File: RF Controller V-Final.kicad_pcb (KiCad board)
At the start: 2 copper layers, 132 x 67.5 mm, 38 parts, among them J2 J_OLED, J3 BAT+, J4 BAT-, SW1 EG1218, U1 Teensy4.0, U3 NRF24L01, U5 AP2112K-3.3, U7 Pitch/Roll, U8 TPS542025DDCR, U9 Throttle/Yaw

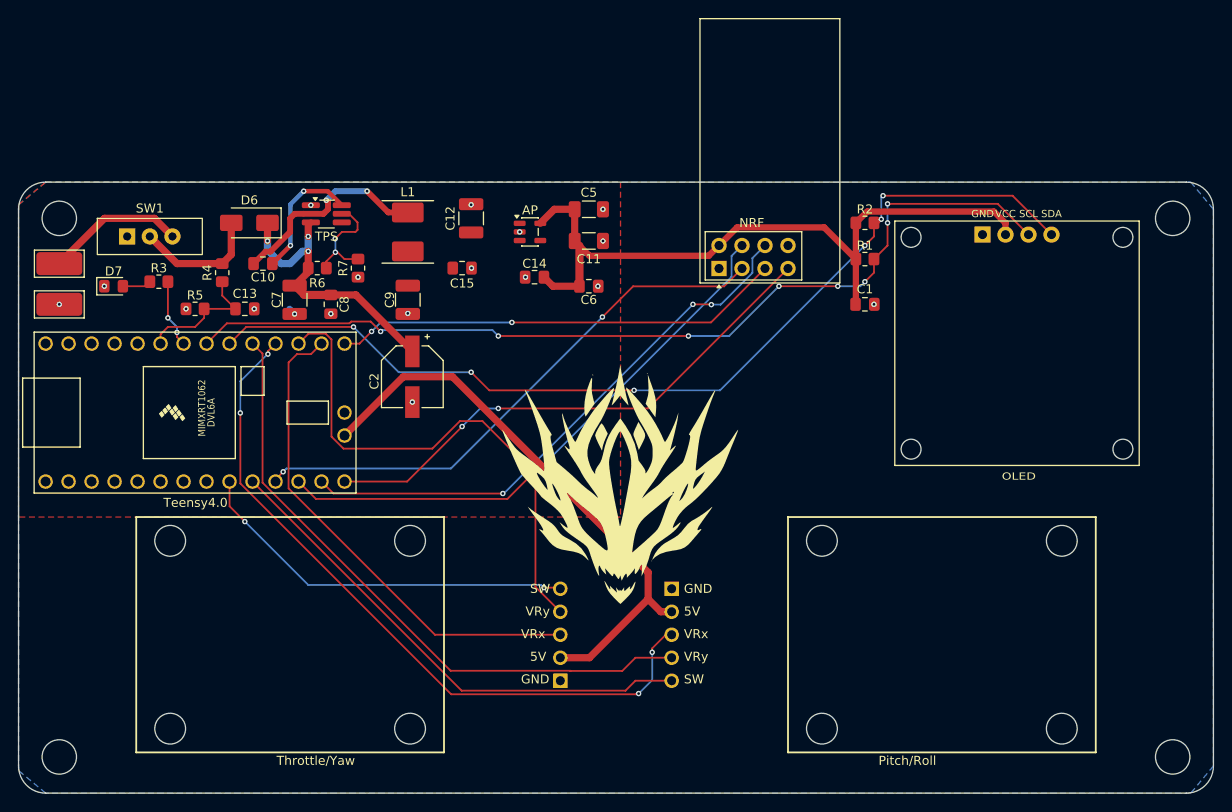
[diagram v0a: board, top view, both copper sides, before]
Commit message: Edited positions
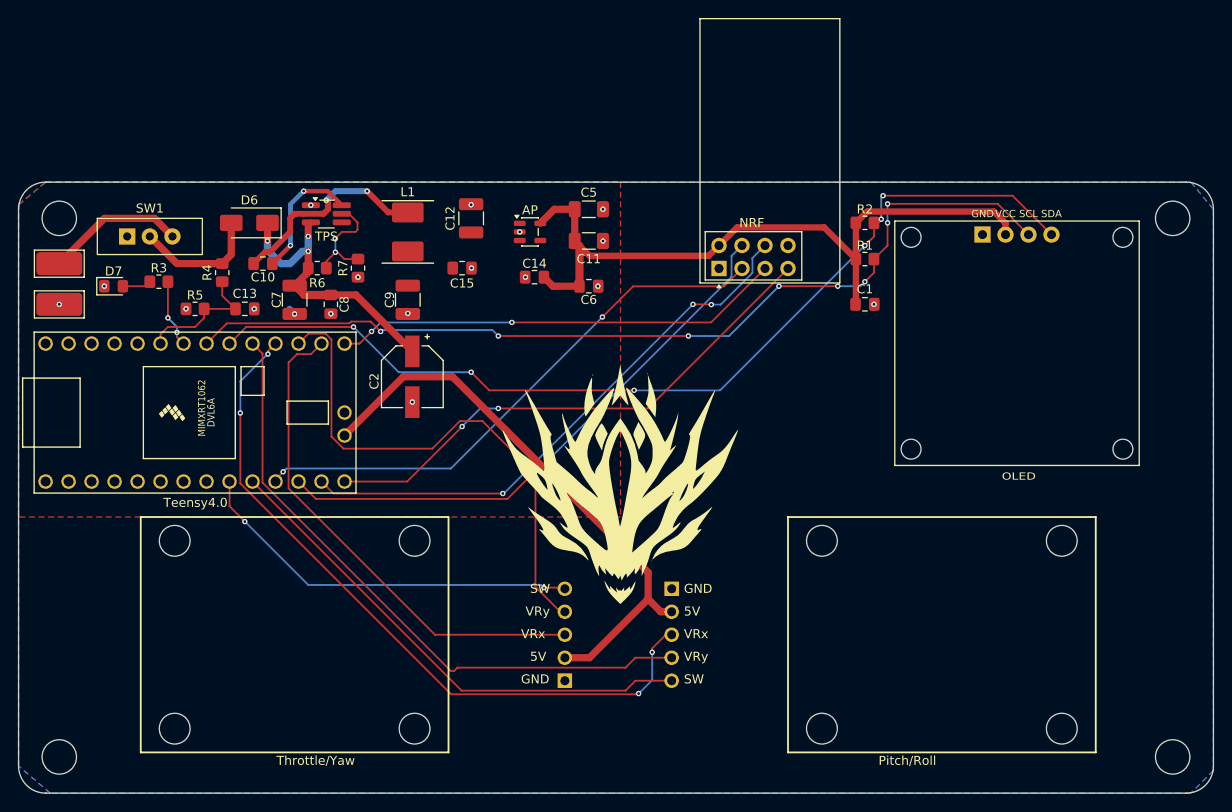
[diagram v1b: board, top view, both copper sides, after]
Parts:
- moved U9 0.50 mm to (129.5, 105.0)
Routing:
- net /D9: track 43.0 -> 44.0 mm
- net /3v3: track 63.7 -> 63.2 mm
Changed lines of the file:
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@@
 	(footprint "JOYYFOOT:JOY1"
 		(layer "F.Cu")
-		(at 129 105 180)
+		(at 129.5 105 180)
 		(property "Reference" "U9"
 			(at 10.73 -10.66 180)
@@
 	)
 	(segment
-		(start 140.039265 112.800735)
-		(end 141.730735 112.800735)
+		(start 142.35 112.92)
+		(end 141.85 112.92)
+		(width 0.2)
+		(layer "F.Cu")
+		(net "/D9")
+	)
+	(segment
+		(start 142.230735 112.800735)
+		(end 142.35 112.92)
 		(width 0.2)
 		(layer "F.Cu")
@@
 	)
 	(segment
-		(start 141.730735 112.800735)
-		(end 141.85 112.92)
+		(start 140.039265 112.800735)
+		(end 142.230735 112.800735)
 		(width 0.2)
 		(layer "F.Cu")
@@
 	)
 	(segment
-		(start 151.55 114.06)
-		(end 145.07 120.54)
-		(width 0.8)
-		(layer "F.Cu")
-		(net "/3v3")
-	)
-	(segment
 		(start 151.55 111.1125)
 		(end 129.9375 89.5)
@@
 	)
 	(segment
-		(start 145.07 120.54)
-		(end 141.85 120.54)
+		(start 151.55 114.06)
+		(end 145.07 120.54)
 		(width 0.8)
 		(layer "F.Cu")
@@
 	)
 	(segment
+		(start 145.07 120.54)
+		(end 142.35 120.54)
+		(width 0.8)
+		(layer "F.Cu")
+		(net "/3v3")
+	)
+	(segment
 		(start 119.66 85.84)
 		(end 118.01 85.84)
@@
 	)
 	(segment
-		(start 128 118)
-		(end 141.85 118)
+		(start 114.31 87)
+		(end 112.754365 87)
 		(width 0.2)
 		(layer "F.Cu")
@@
 	)
 	(segment
-		(start 112.754365 87)
-		(end 114.31 87)
+		(start 111.83 87.924365)
+		(end 111.83 101.83)
 		(width 0.2)
 		(layer "F.Cu")
@@
 	)
 	(segment
-		(start 111.83 87.924365)
-		(end 112.754365 87)
+		(start 115.47 85.84)
+		(end 114.31 87)
 		(width 0.2)
 		(layer "F.Cu")
@@
 	)
 	(segment
-		(start 111.83 101.83)
-		(end 111.83 87.924365)
+		(start 128 118)
+		(end 142.35 118)
 		(width 0.2)
 		(layer "F.Cu")
@@
 	)
 	(segment
-		(start 114.31 87)
-		(end 115.47 85.84)
+		(start 112.754365 87)
+		(end 111.83 87.924365)
 		(width 0.2)
 		(layer "F.Cu")
@@
 	)
 	(segment
-		(start 128 118)
-		(end 111.83 101.83)
+		(start 111.83 101.83)
+		(end 128 118)
 		(width 0.2)
 		(layer "F.Cu")
@@
 	)
 	(segment
-		(start 116.57 85.384365)
-		(end 116.57 96.115635)
+		(start 127.711471 97.44)
+		(end 130.751471 94.4)
 		(width 0.2)
 		(layer "F.Cu")
@@
 	(segment
 		(start 139.1 112.71)
-		(end 141.85 115.46)
+		(end 141.545 115.155)
 		(width 0.2)
 		(layer "F.Cu")
@@
 	)
 	(segment
-		(start 114.03 84.74)
-		(end 115.925635 84.74)
+		(start 139.1 100.251471)
+		(end 139.1 112.71)
 		(width 0.2)
 		(layer "F.Cu")
@@
 	)
 	(segment
-		(start 141.85 115.155)
-		(end 141.85 115.46)
+		(start 141.545 115.155)
+		(end 141.85 115.155)
 		(width 0.2)
 		(layer "F.Cu")
@@
 	)
 	(segment
-		(start 117.894365 97.44)
-		(end 127.711471 97.44)
+		(start 133.248529 94.4)
+		(end 139.1 100.251471)
 		(width 0.2)
 		(layer "F.Cu")
@@
 	)
 	(segment
-		(start 116.57 96.115635)
-		(end 117.894365 97.44)
+		(start 114.03 84.74)
+		(end 115.925635 84.74)
 		(width 0.2)
 		(layer "F.Cu")
@@
 	)
 	(segment
-		(start 127.711471 97.44)
-		(end 130.751471 94.4)
+		(start 115.925635 84.74)
+		(end 116.57 85.384365)
 		(width 0.2)
 		(layer "F.Cu")
@@
 	)
 	(segment
-		(start 139.1 100.251471)
-		(end 139.1 112.71)
+		(start 116.57 85.384365)
+		(end 116.57 96.115635)
 		(width 0.2)
 		(layer "F.Cu")
@@
 	)
 	(segment
-		(start 115.925635 84.74)
-		(end 116.57 85.384365)
+		(start 117.894365 97.44)
+		(end 127.711471 97.44)
 		(width 0.2)
 		(layer "F.Cu")
@@
 	)
 	(segment
-		(start 133.248529 94.4)
-		(end 139.1 100.251471)
+		(start 116.57 96.115635)
+		(end 117.894365 97.44)
 		(width 0.2)
 		(layer "F.Cu")
@@
 	)
 	(segment
-		(start 129.734365 121.98)
-		(end 108.95 101.195635)
+		(start 107.85 85.84)
+		(end 108.95 86.94)
 		(width 0.2)
 		(layer "F.Cu")
@@
 	)
 	(segment
-		(start 154.15 120.54)
-		(end 150.15 120.54)
+		(start 108.95 86.94)
+		(end 108.95 101.195635)
 		(width 0.2)
 		(layer "F.Cu")
@@
 	)
 	(segment
-		(start 142.97 122)
-		(end 142.95 121.98)
+		(start 150.15 120.54)
+		(end 154.15 120.54)
 		(width 0.2)
 		(layer "F.Cu")
@@
 	)
 	(segment
-		(start 108.95 86.94)
-		(end 107.85 85.84)
+		(start 130.474365 121.64)
+		(end 149.05 121.64)
 		(width 0.2)
 		(layer "F.Cu")
@@
 	)
 	(segment
-		(start 150.15 120.54)
-		(end 148.69 122)
+		(start 129.754365 122)
+		(end 130.114365 122)
 		(width 0.2)
 		(layer "F.Cu")
@@
 	)
 	(segment
-		(start 142.95 121.98)
-		(end 129.734365 121.98)
+		(start 149.05 121.64)
+		(end 150.15 120.54)
 		(width 0.2)
 		(layer "F.Cu")
@@
 	(segment
 		(start 108.95 101.195635)
-		(end 108.95 86.94)
+		(end 129.754365 122)
 		(width 0.2)
 		(layer "F.Cu")
@@
 	)
 	(segment
-		(start 148.69 122)
-		(end 142.97 122)
+		(start 130.114365 122)
+		(end 130.474365 121.64)
 		(width 0.2)
 		(layer "F.Cu")
@@
 		(polygon
 			(pts
-				(xy 82 70.5) (xy 85 68) (xy 211.5 68) (xy 214 71) (xy 214 132.5) (xy 211.5 135.5) (xy 85 135.5)
-				(xy 82 133)
+				(xy 82 70.5) (xy 85 68) (xy 211.5 68) (xy 214 71) (xy 214 133) (xy 211.5 135.5) (xy 85.5 135.5)
+				(xy 82 132.5)
 			)
 		)
